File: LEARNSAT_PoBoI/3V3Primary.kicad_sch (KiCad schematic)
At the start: 17 parts, among them Q901 SI7164DP-T1-GE3, Q902 SI5418DU-T1-GE3, U901 INA219AIDCNR, U902 LTC4231IUD-2#TRPBF

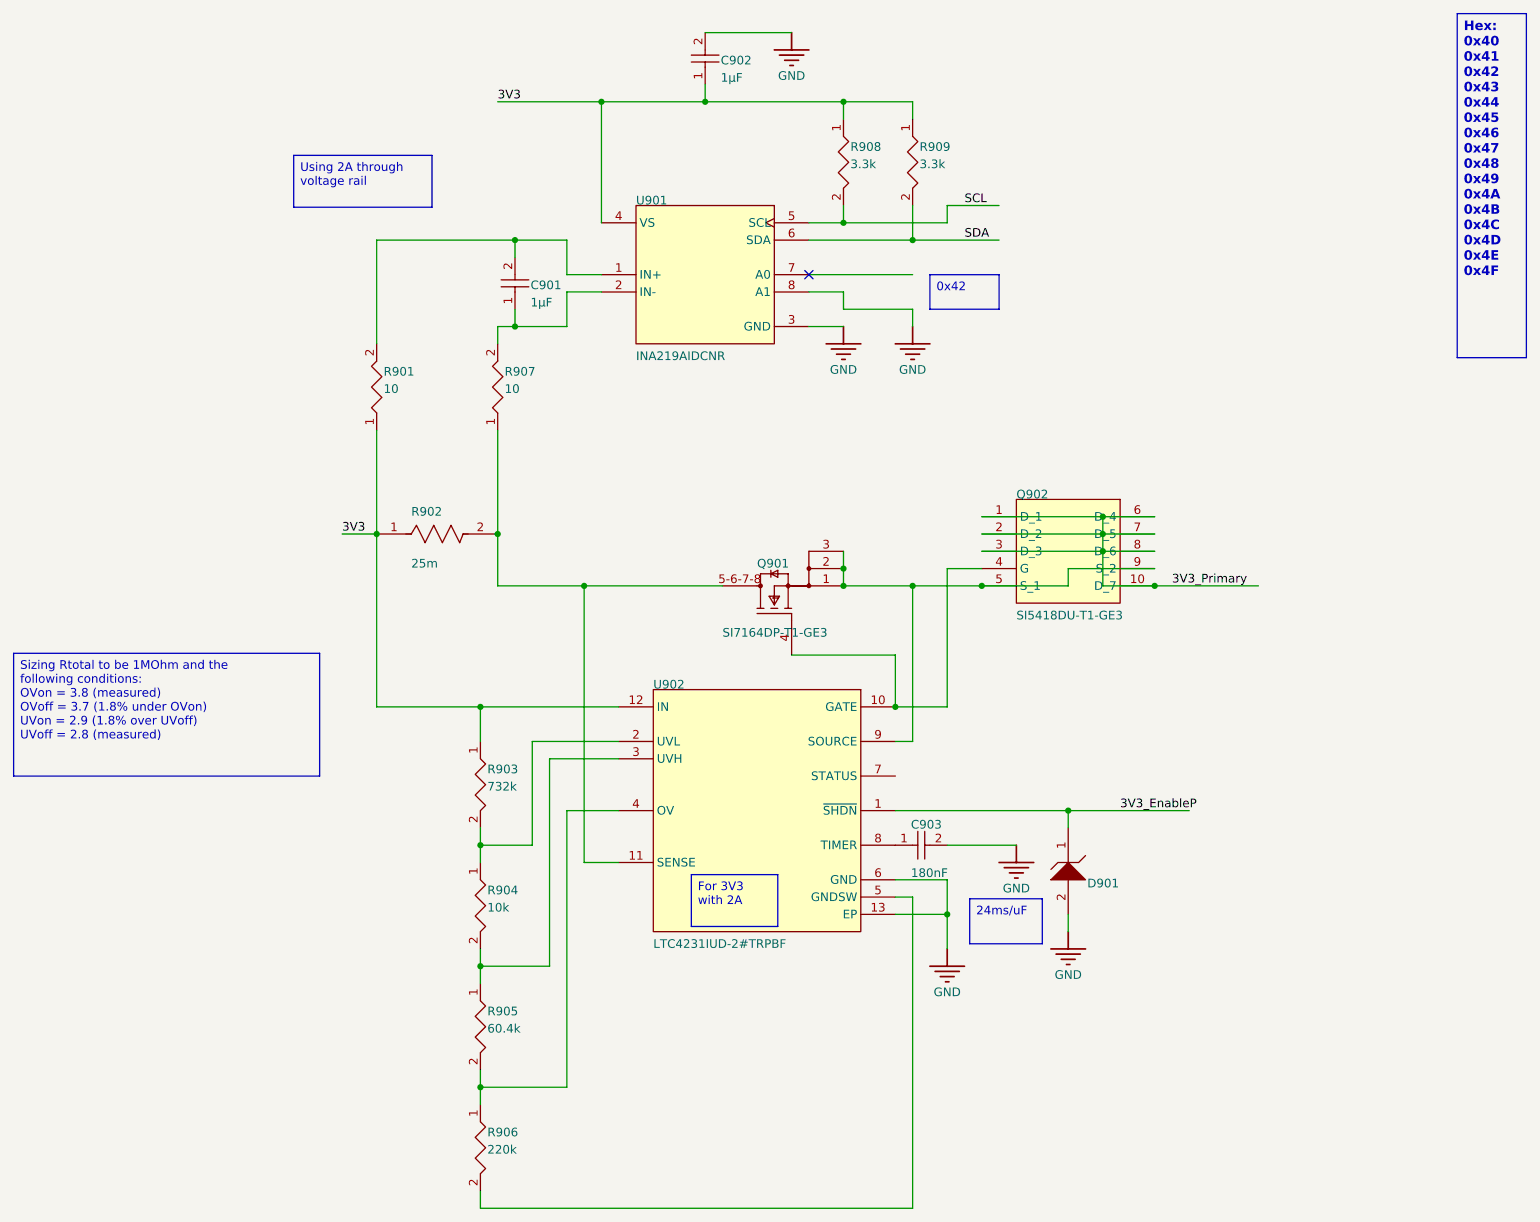
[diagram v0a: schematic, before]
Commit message: Add files via upload
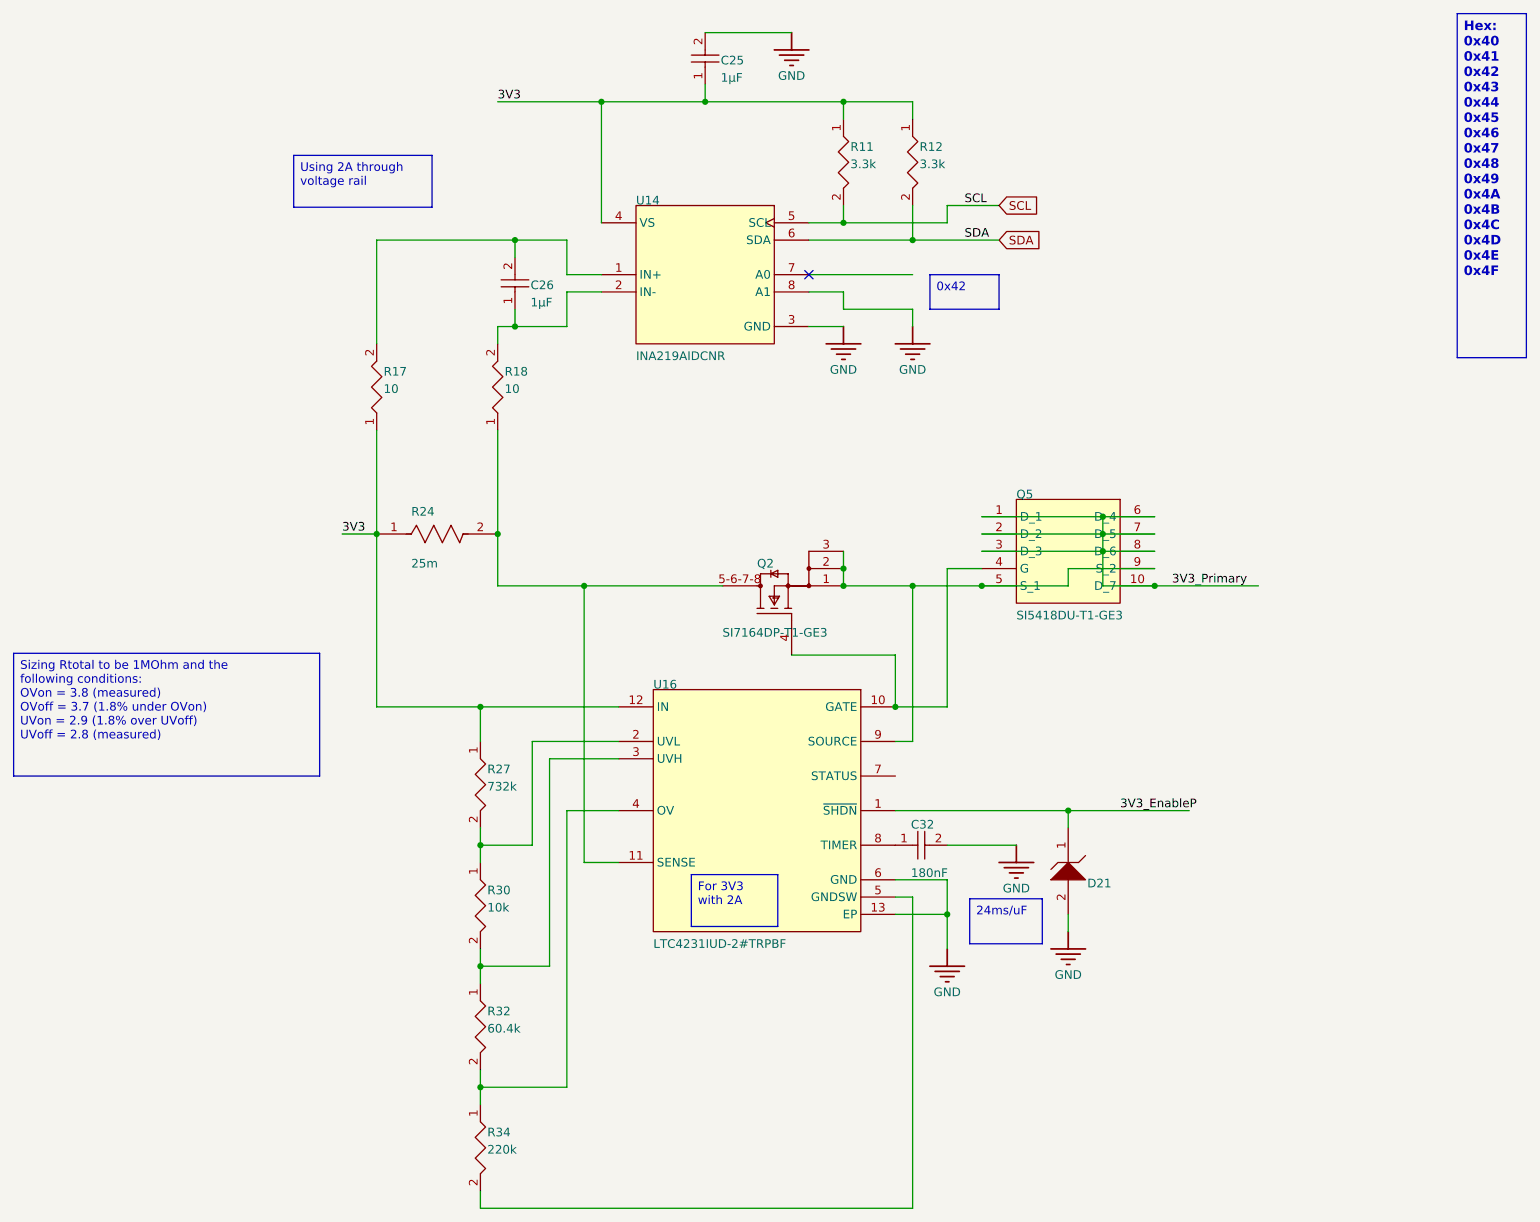
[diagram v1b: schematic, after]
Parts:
- C25: renamed from C902; footprint Capacitor_SMD:C_0603_1608Metric -> CAPC1608X90X35ML15T15
- C26: renamed from C901; footprint Capacitor_SMD:C_0603_1608Metric -> CAPC1608X90X40LL10T20
- C32: renamed from C903; footprint Capacitor_SMD:C_0805_2012Metric -> FP-C0805C-DN-IPC_A
- D21: renamed from D901; footprint Diode_SMD:D_SOD-323 -> ONSC-SOD-323-2-477-02_V
- Q2: renamed from Q901; footprint Package_SO:Vishay_PowerPAK_1212-8_Single -> Vishay_S17-0173-SINGLE_MFG
- Q5: renamed from Q902; footprint Package_SO:Vishay_PowerPAK_1212-8_Single -> SI5418DU-T1-GE3-Footprint-1
- R11: renamed from R908; footprint Resistor_SMD:R_1210_3225Metric -> FP-CRCW1210-e3-IPC_C
- R12: renamed from R909; footprint Resistor_SMD:R_1210_3225Metric -> FP-CRCW1210-e3-IPC_C
- R17: renamed from R901; footprint Resistor_SMD:R_0402_1005Metric -> RESC0402(1005)_L
- R18: renamed from R907; footprint Resistor_SMD:R_0402_1005Metric -> RESC0402(1005)_L
- R24: renamed from R902; footprint Resistor_SMD:R_1206_3216Metric -> FP-CSR1206-IPC_C
- R27: renamed from R903; footprint Resistor_SMD:R_0805_2012Metric -> FP-CR0805-IPC_A
- R30: renamed from R904; footprint Resistor_SMD:R_0402_1005Metric -> RESC1005X40X25ML05T05
- R32: renamed from R905; footprint Resistor_SMD:R_0402_1005Metric -> RESC1005X40X25NL05T10
- R34: renamed from R906; footprint Resistor_SMD:R_0402_1005Metric -> FP-ESR01-IPC_C
- U14: renamed from U901; footprint INA219AIDCNR:SOT65P280X145-8N -> FP-DCN0008A-IPC_A
- U16: renamed from U902; footprint LTC4231IUD-2_TRPBF:QFN50P300X300X80-13N -> FP-UD-12-05-08-1855-IPC_A

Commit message: Added footprints
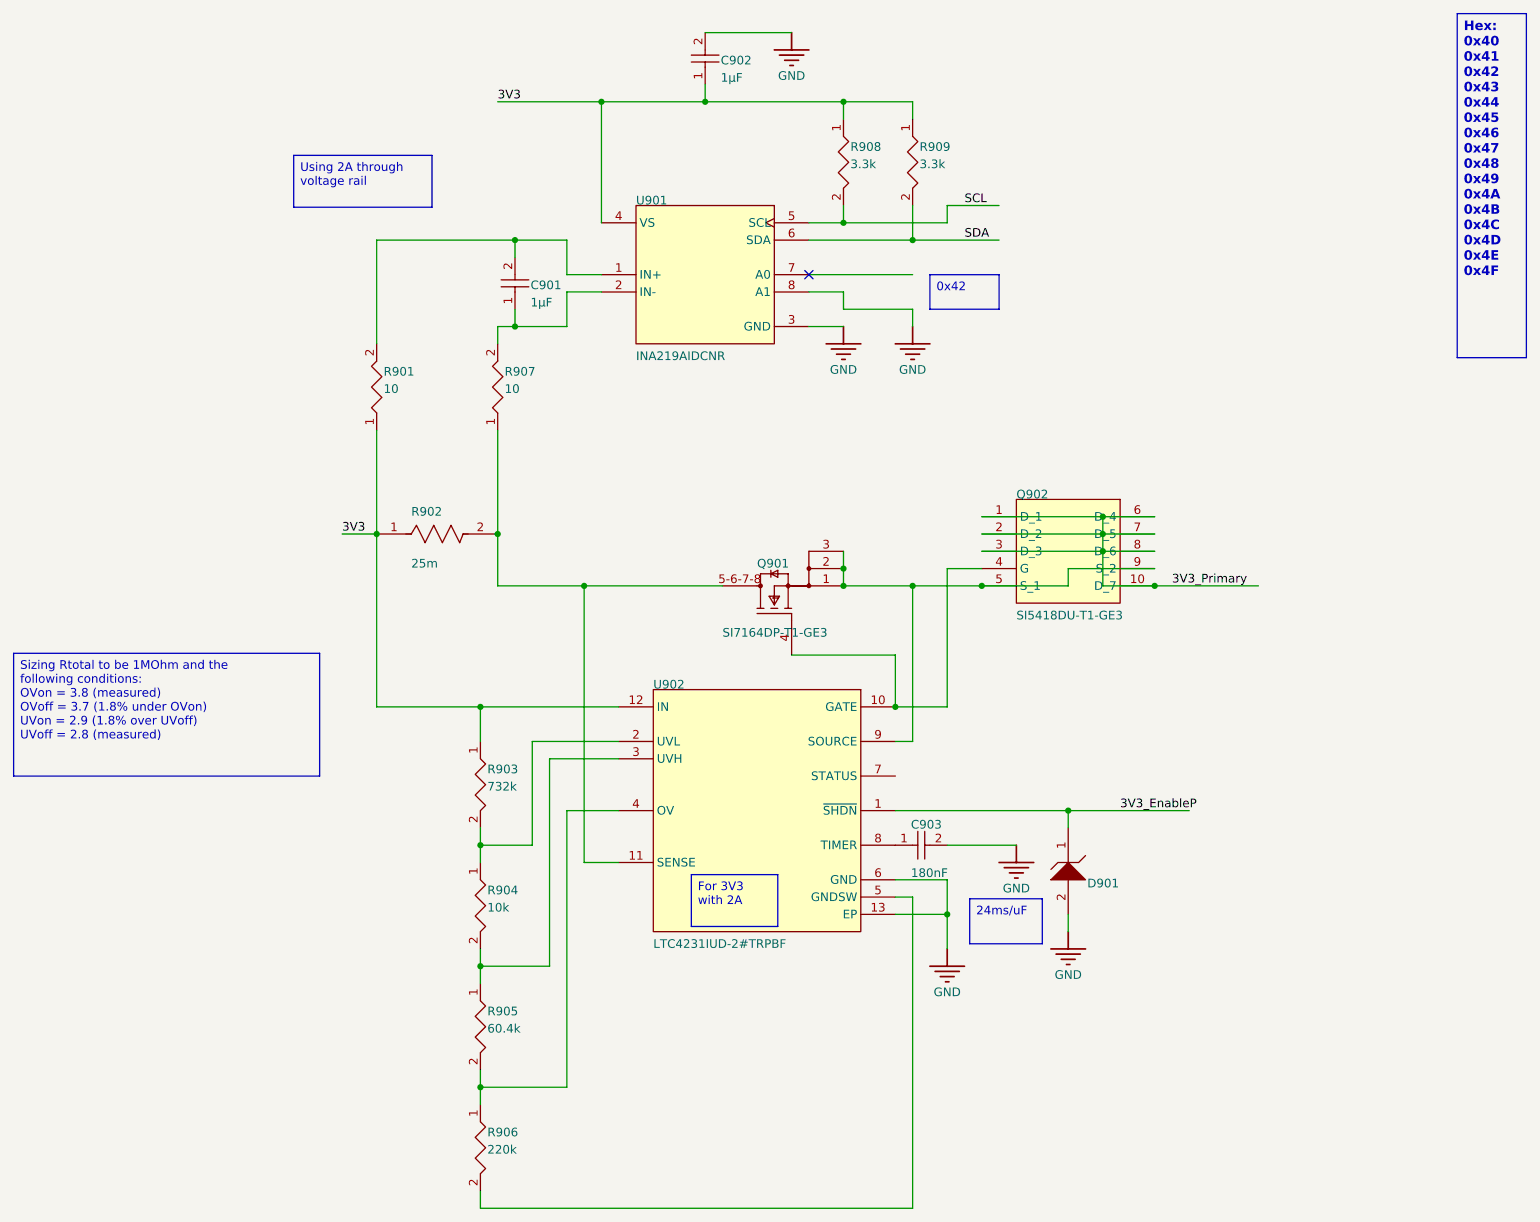
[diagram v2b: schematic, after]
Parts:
- C901: renamed from C26; footprint CAPC1608X90X40LL10T20 -> Capacitor_SMD:C_0603_1608Metric
- C902: renamed from C25; footprint CAPC1608X90X35ML15T15 -> Capacitor_SMD:C_0603_1608Metric
- C903: renamed from C32; footprint FP-C0805C-DN-IPC_A -> Capacitor_SMD:C_0805_2012Metric
- D901: renamed from D21; footprint ONSC-SOD-323-2-477-02_V -> Diode_SMD:D_SOD-323
- Q901: renamed from Q2; footprint Vishay_S17-0173-SINGLE_MFG -> Package_SO:Vishay_PowerPAK_1212-8_Single
- Q902: renamed from Q5; footprint SI5418DU-T1-GE3-Footprint-1 -> Package_SO:Vishay_PowerPAK_1212-8_Single
- R901: renamed from R17; footprint RESC0402(1005)_L -> Resistor_SMD:R_0402_1005Metric
- R902: renamed from R24; footprint FP-CSR1206-IPC_C -> Resistor_SMD:R_1206_3216Metric
- R903: renamed from R27; footprint FP-CR0805-IPC_A -> Resistor_SMD:R_0805_2012Metric
- R904: renamed from R30; footprint RESC1005X40X25ML05T05 -> Resistor_SMD:R_0402_1005Metric
- R905: renamed from R32; footprint RESC1005X40X25NL05T10 -> Resistor_SMD:R_0402_1005Metric
- R906: renamed from R34; footprint FP-ESR01-IPC_C -> Resistor_SMD:R_0402_1005Metric
- R907: renamed from R18; footprint RESC0402(1005)_L -> Resistor_SMD:R_0402_1005Metric
- R908: renamed from R11; footprint FP-CRCW1210-e3-IPC_C -> Resistor_SMD:R_1210_3225Metric
- R909: renamed from R12; footprint FP-CRCW1210-e3-IPC_C -> Resistor_SMD:R_1210_3225Metric
- U901: renamed from U14; footprint FP-DCN0008A-IPC_A -> INA219AIDCNR:SOT65P280X145-8N
- U902: renamed from U16; footprint FP-UD-12-05-08-1855-IPC_A -> LTC4231IUD-2_TRPBF:QFN50P300X300X80-13N
